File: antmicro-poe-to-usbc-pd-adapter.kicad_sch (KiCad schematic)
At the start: 93 parts, among them J1 Bus_RJ45_5-2337992-8, J2 Bus_RJ45_5-2337992-8, J3 USB-C_GCT_USB4105-GF-A, Q1 PJE138K, U1 TPS2372-3RGWR, U2 LV14540DDAR, U3 INA230AIRGTR, U4 IEA48003A280V-001-R, U5 FT4232H_VQFN, U6 TPS65987DDHRSHR, U7 LV14540DDAR, Y1 Resonator_12MHz_ABM8G

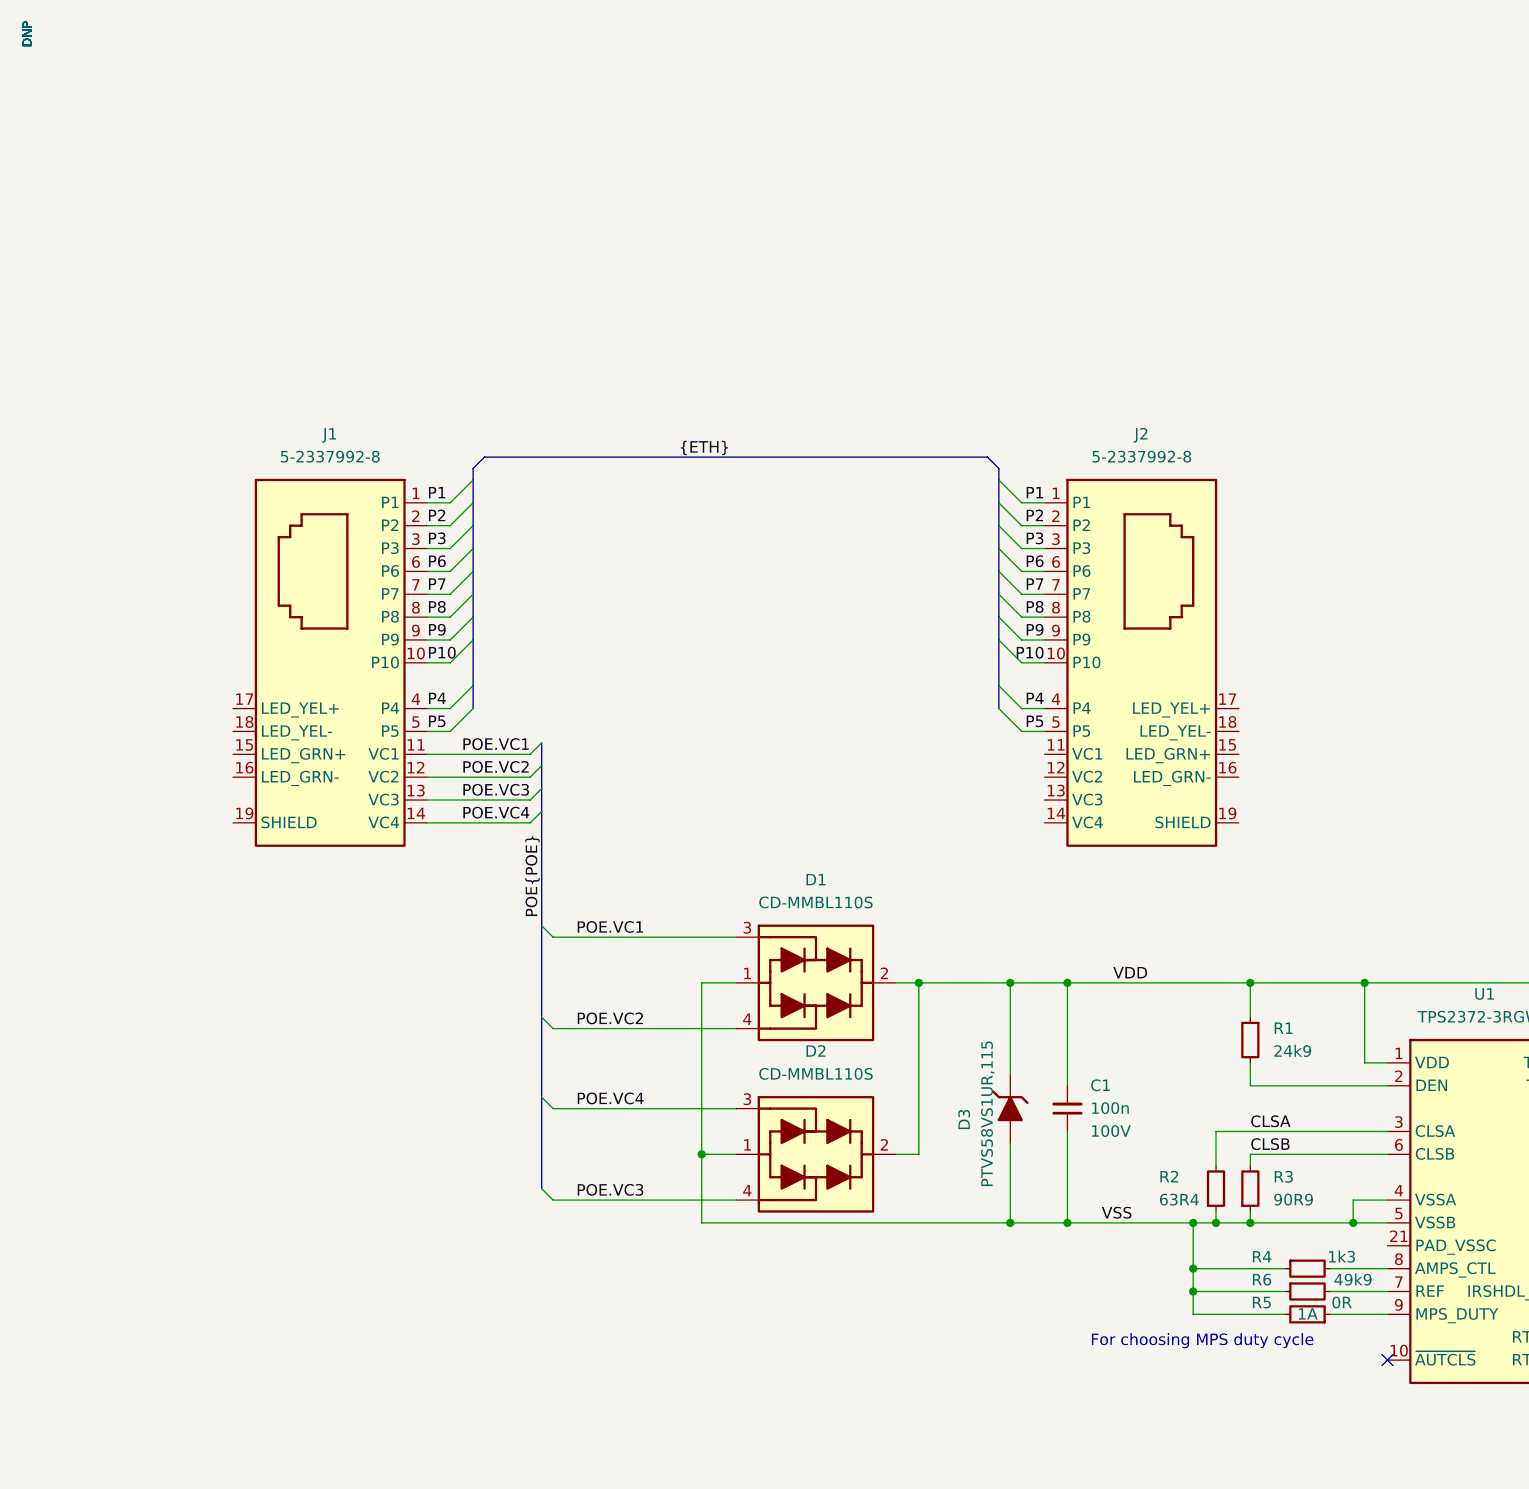
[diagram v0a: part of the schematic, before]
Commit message: [#62182] Update resistor fields
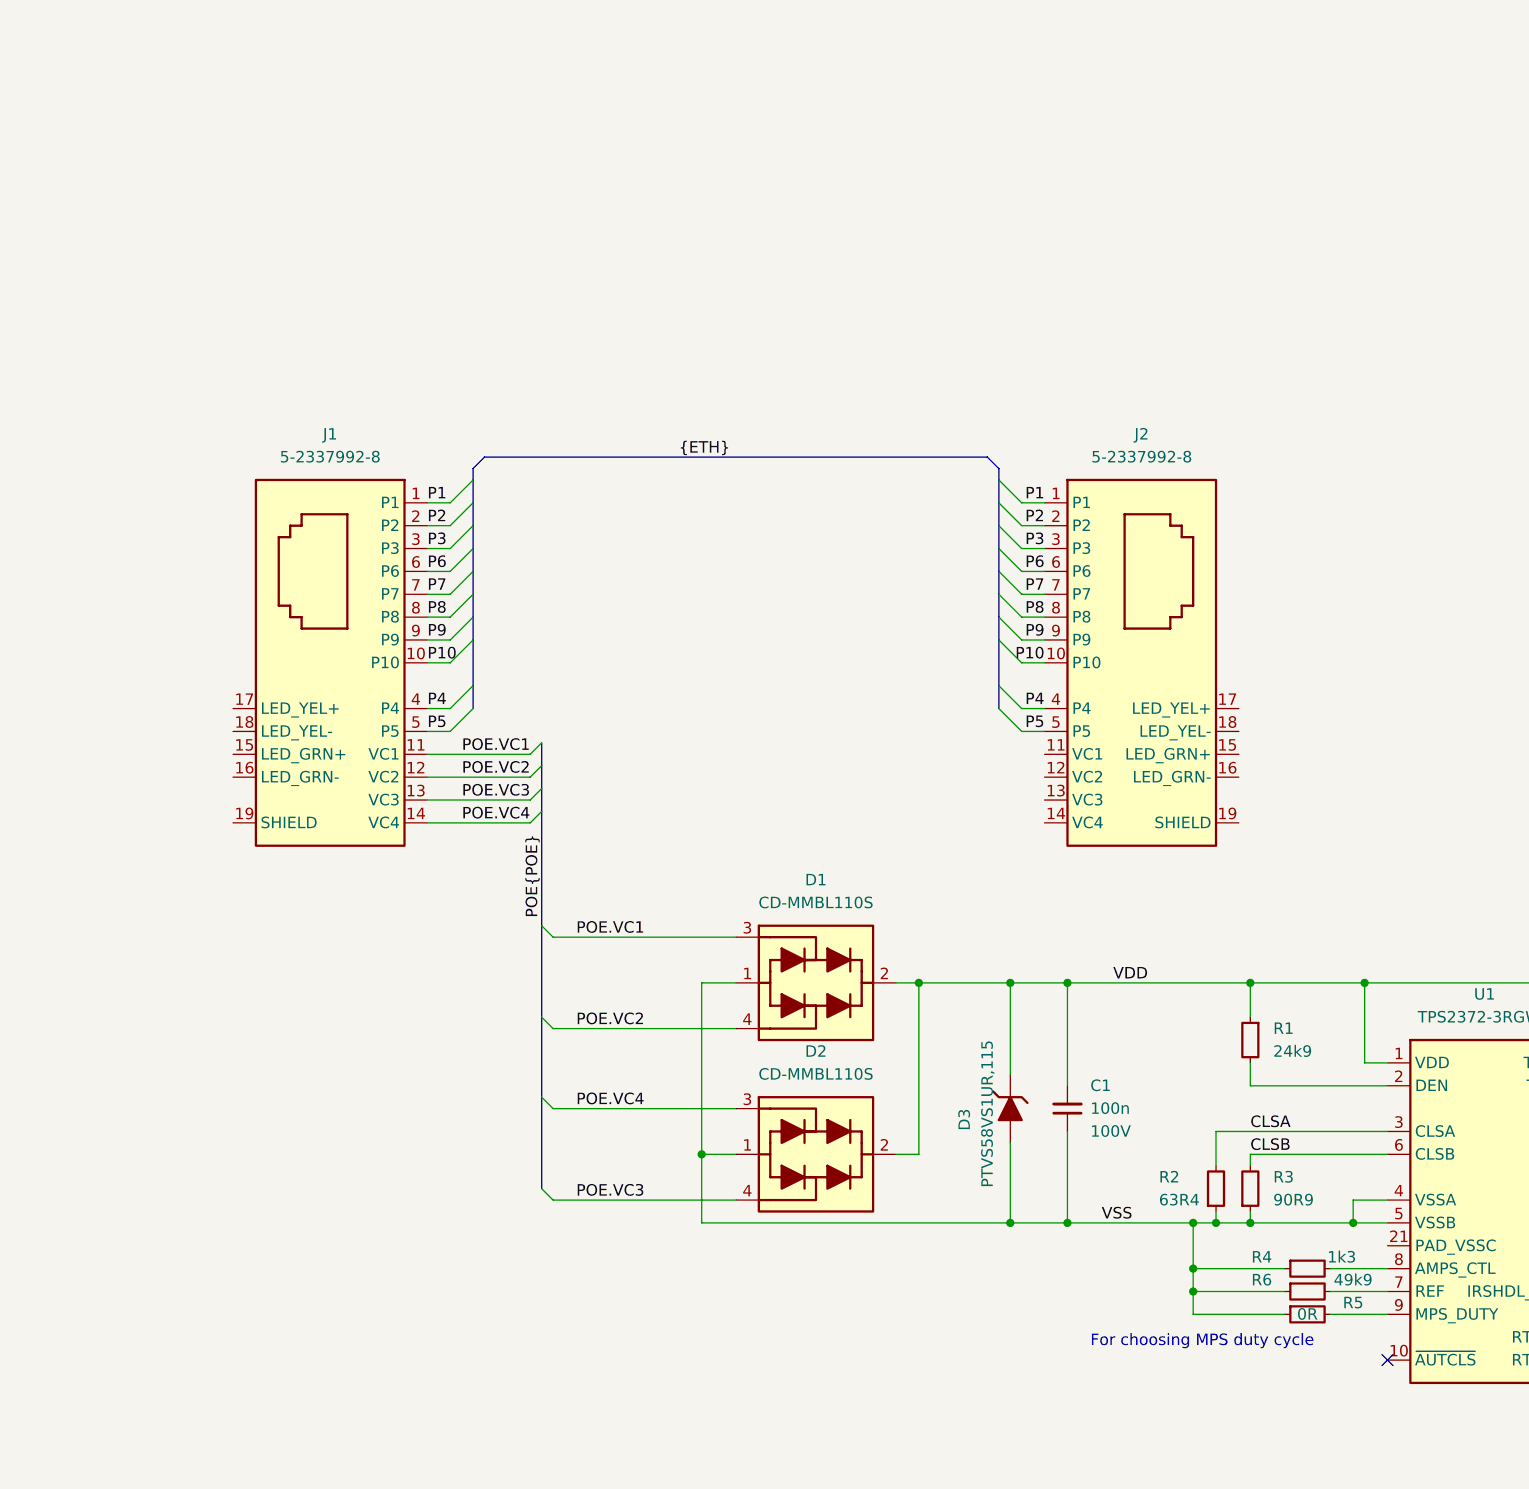
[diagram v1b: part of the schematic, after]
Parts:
- C2, R33, R34, R35, R36, R37, R38, R39, R40: DNP DNP -> (none); now in the parts list
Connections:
- net VSS: now also R5.1; no longer R5.2
- net at U1.9 (MPS_DUTY): now also R5.2; no longer R5.1
